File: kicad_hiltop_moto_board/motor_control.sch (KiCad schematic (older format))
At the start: 32 parts, among them Q1 CSD18540Q5B, Q2 CSD18540Q5B, Q3 CSD18540Q5B, Q4 CSD18540Q5B, Q5 CSD18540Q5B, Q6 CSD18540Q5B, Q7 CSD18540Q5B, Q8 CSD18540Q5B, U1 DRV8704

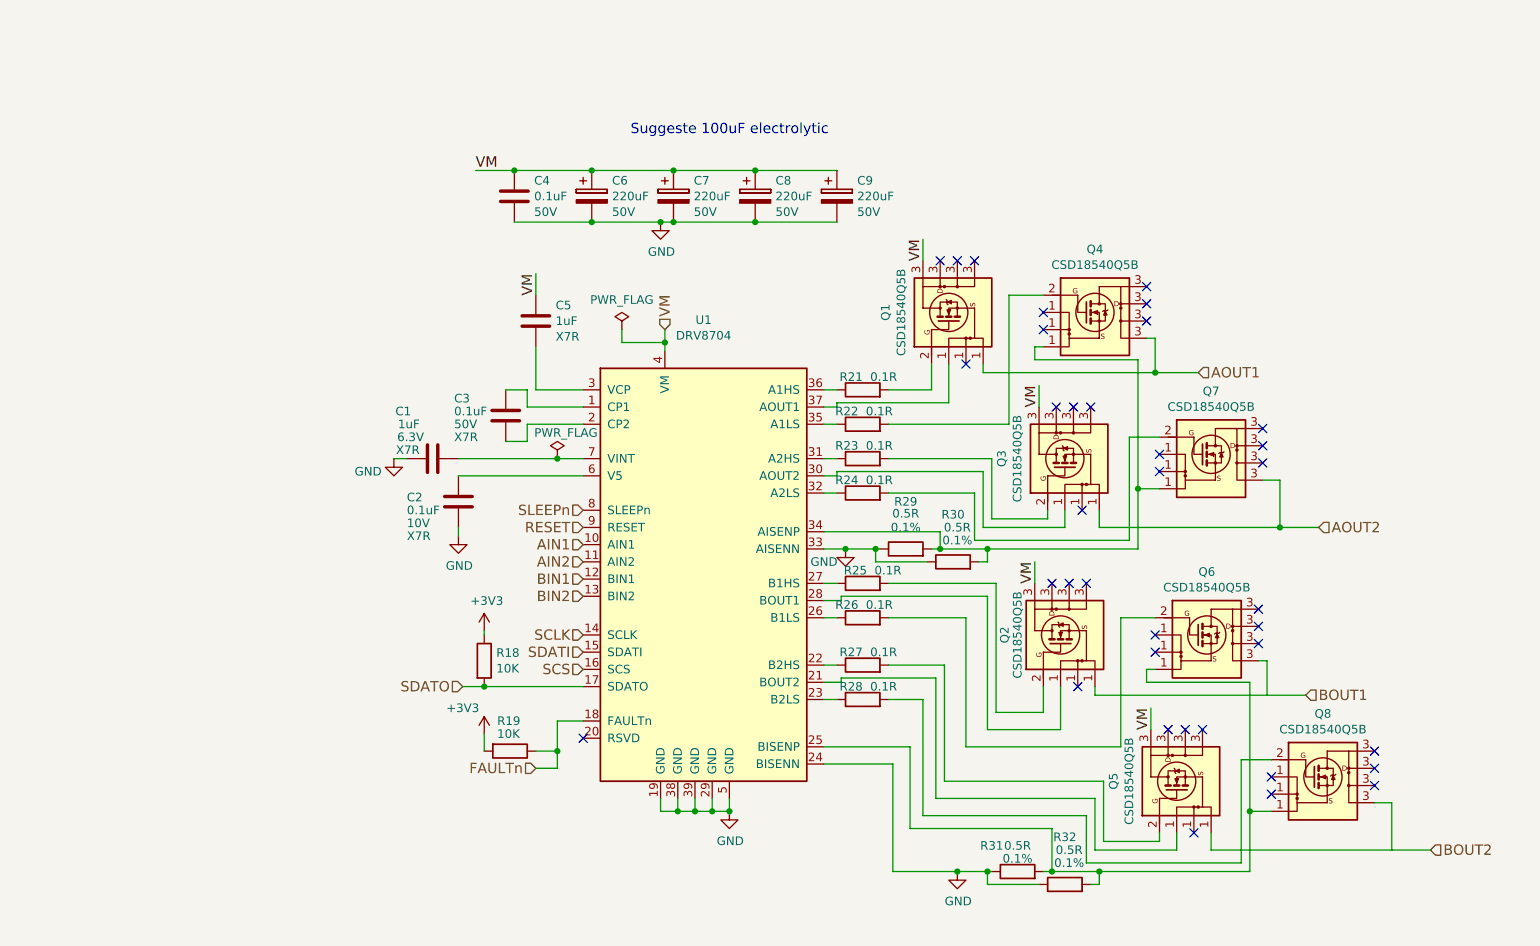
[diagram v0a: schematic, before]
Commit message: Started on moto board layout
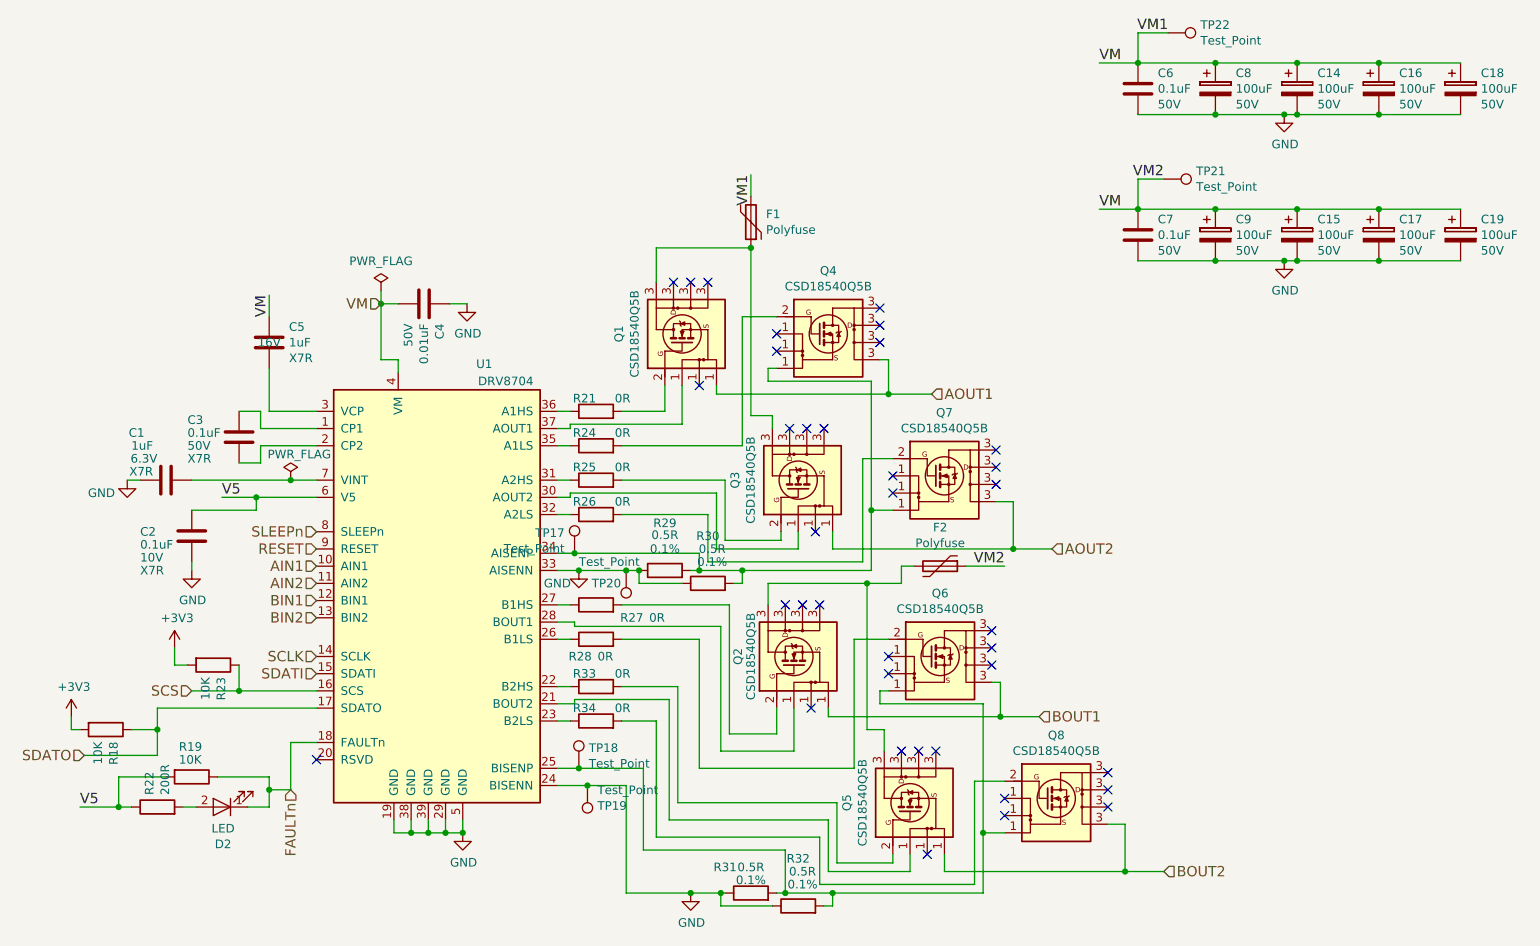
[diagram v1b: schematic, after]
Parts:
- removed C6, C7: 220uF, symbol device:CP
- added C14, C15, C16, C17, C18, C19: 100uF, Capacitor_SMD:CP_Elec_6.3x7.7, symbol device:CP
- added C6, C7: 0.1uF, Capacitor_SMD:C_0402_1005Metric, symbol device:C
- added D2: LED, LED_SMD:LED_0603_1608Metric, symbol device:LED
- added F1, F2: Polyfuse, Fuse:Fuse_2920_7451Metric, symbol device:Polyfuse
- added R33, R34: 0R, Resistor_SMD:R_0603_1608Metric, symbol device:R
- added TP17, TP18, TP19, TP20, TP21, TP22: Test_Point, TestPoint:TestPoint_THTPad_D1.0mm_Drill0.5mm, symbol Connector:Test_Point
- C1, C2, C3, C5: footprint (none) -> Capacitor_SMD:C_0402_1005Metric
- C4: value 0.1uF -> 0.01uF; footprint (none) -> Capacitor_SMD:C_0402_1005Metric
- C8, C9: value 220uF -> 100uF; footprint (none) -> Capacitor_SMD:CP_Elec_6.3x7.7
- Q1, Q2, Q3, Q4, Q5, Q6, Q7, Q8: footprint TO_SOT_Packages_SMD:TDSON-8-1 -> Package_SON:VSONP-8-1EP_5x6_P1.27mm
- R18, R19, R29, R30, R31, R32: footprint (none) -> Resistor_SMD:R_0603_1608Metric
- R21, R24, R25, R26, R27, R28: value 0.1R -> 0R; footprint (none) -> Resistor_SMD:R_0603_1608Metric
- R22: value 0.1R -> 200R; footprint (none) -> Resistor_SMD:R_0603_1608Metric
- R23: value 0.1R -> 10K; footprint (none) -> Resistor_SMD:R_0603_1608Metric
- U1: footprint (none) -> Devtank_PCB_Lib:DRV8704
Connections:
- net +3V3: now also R18.2, R23.2; no longer R18.1, R19.2
- net FAULTn: now also D2.1 (K)
- net GND: now also C4.1, C14.2, C15.2, C16.2, C17.2, C18.2, C19.2, C6.2, C7.2, TP19.1, TP20.1; no longer C4.2
- net SCS: now also R23.1
- net SDATO: now also R18.1; no longer R18.2
- net VM: now also C4.2, C14.1, C15.1, C16.1, C17.1, C18.1, C19.1, C6.1, C7.1, F1.2, F2.1, TP21.1, TP22.1; no longer C4.1, Q1.3 (D), Q2.3 (D), Q3.3 (D), Q5.3 (D)
- net at R27.1: now also U1.27 (B1HS); no longer U1.22 (B2HS)
- net at R28.1: now also U1.26 (B1LS); no longer U1.23 (B2LS)
- net at Q6.1 (S), Q8.1 (S), R31.2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: now also TP18.1
- net at R26.1: now also U1.32 (A2LS); no longer U1.26 (B1LS)
- net at R25.1: now also U1.31 (A2HS); no longer U1.27 (B1HS)
- net at R24.1: now also U1.35 (A1LS); no longer U1.32 (A2LS)
- net at Q4.1 (S), Q7.1 (S), R29.2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: now also TP17.1
- net V5: now reaches R22.1
- net V5: now also C2.1, R19.2, U1.6 (V5); no longer U1.35 (A1LS)
- net at R22.2: now also D2.2 (A); no longer Q4.2 (G)
- net at Q3.2 (G): now also R25.2; no longer R23.2
- net at R24.2: now also Q4.2 (G); no longer Q7.2 (G)
- net at Q2.2 (G): now also R27.2; no longer R25.2
- net at R26.2: now also Q7.2 (G); no longer Q6.2 (G)
- net at Q5.2 (G): now also R33.2; no longer R27.2
- net at R28.2: now also Q6.2 (G); no longer Q8.2 (G)
- new net: F1.1, Q1.3 (D), Q3.3 (D)
- new net: F2.2, Q2.3 (D), Q5.3 (D)
- new net: R33.1, U1.22 (B2HS)
- new net: R34.1, U1.23 (B2LS)
- new net: Q8.2 (G), R34.2
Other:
- note removed: "Suggeste 100uF electrolytic\n"
- moved on the sheet: C1, C2, C3, C4, C5, Q1, Q2, Q3, Q4, Q5, Q6, Q7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
